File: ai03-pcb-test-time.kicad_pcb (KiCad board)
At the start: 2 copper layers, 24 parts, among them SW1 SW_Push, U1 ATmega32U4-AU, Y1 16MHz

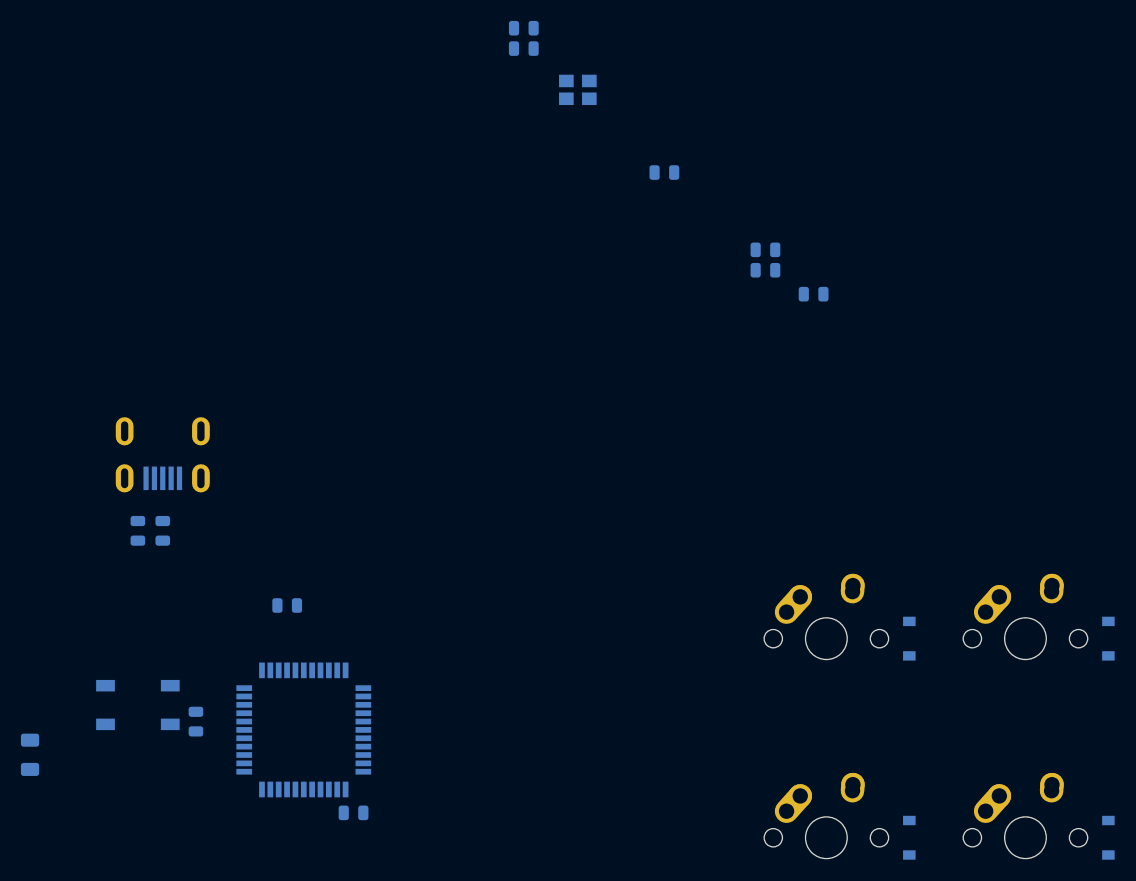
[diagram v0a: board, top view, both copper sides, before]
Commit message: Schleep for real
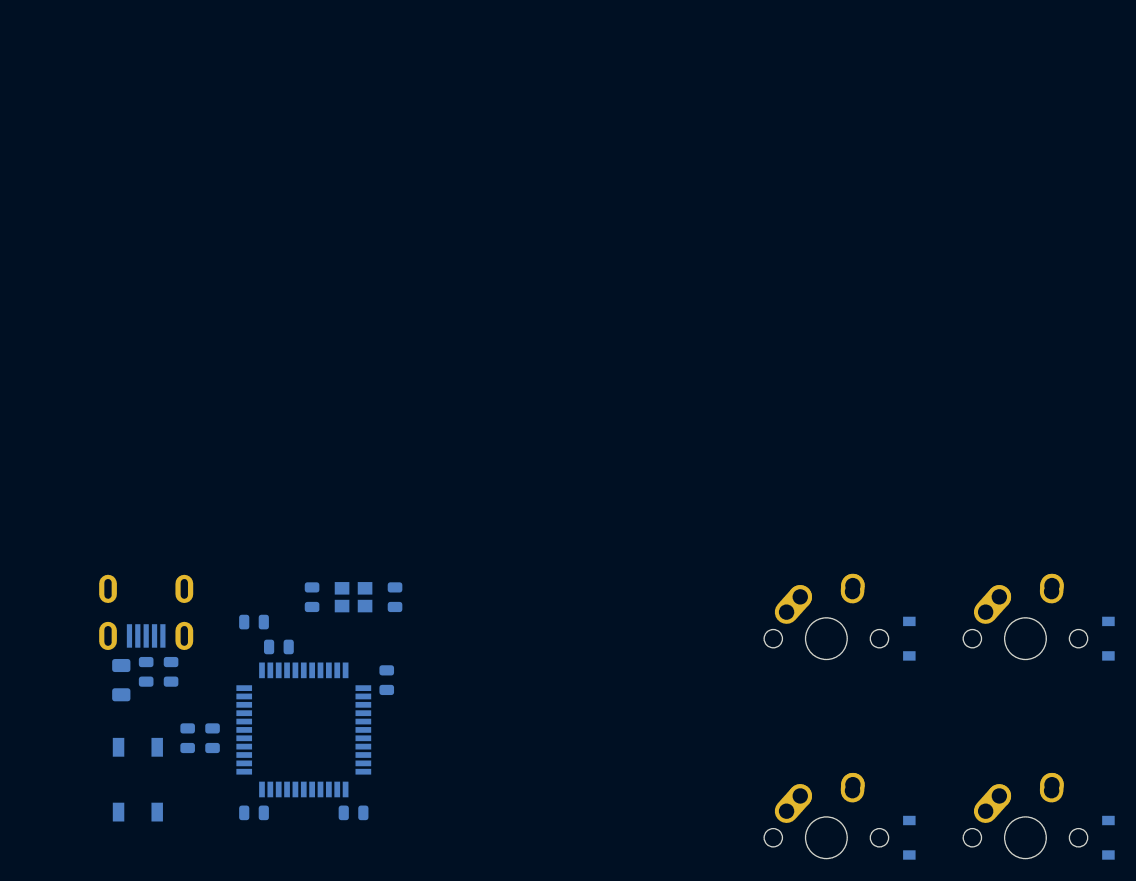
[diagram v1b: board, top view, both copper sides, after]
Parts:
- moved C7 72.8 mm to (42.1, 97.6)
- moved C5 72.4 mm to (35.7, 90.5), turned to 270 degrees
- moved C2 63.7 mm to (44.5, 81.8)
- moved C1 61.8 mm to (54.8, 84.9), turned to 90 degrees
- moved C4 56.1 mm to (47.6, 77.0), turned to 270 degrees
- moved Y1 53.1 mm to (51.6, 77.0), turned to 180 degrees
- moved C3 47.3 mm to (55.6, 77.0), turned to 90 degrees
- moved USB1 15.2 mm to (31.8, 76.2)
- moved R1 13.5 mm to (31.8, 84.1)
- moved R2 13.5 mm to (34.1, 84.1)
- moved F1 11.3 mm to (29.4, 84.9)
- moved SW1 7.14 mm to (31.0, 94.5), turned to 270 degrees
- moved R3 3.55 mm to (42.1, 79.4)
- moved C6 2.25 mm to (38.1, 90.5)
